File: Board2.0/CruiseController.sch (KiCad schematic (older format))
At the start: 56 parts, among them J1 USB_B_Micro, J2 Conn_02x09_Top_Bottom, U1 ADG884, U3 TLV9064IRTER, U5 MIC5225, U6 MCP2562-E-MF, U7 STM32L433CCUx, Y1 32.768

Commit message: udpate v2 pcb
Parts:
- added R22, R23: 75, Resistor_SMD:R_0603_1608Metric, symbol Device:R_Small
- added U2: CPC1017N, Package_SO:SOP-4_3.8x4.1mm_P2.54mm, symbol Relay_SolidState:CPC1017N
- U1: symbol VeridianDesigns:ADG884 -> CruiseController-rescue:ADG884-VeridianDesigns
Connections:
- net GND: now also J2.11 (Pin_11), U2.2; no longer J2.10 (Pin_10)
- net INTERSW: no longer J2.11 (Pin_11)
- net VIN: no longer J2.1 (Pin_1)
- net HZEN: now reaches U7.16 (PA6)
- net HZEN: now also R22.2
- new net: R23.1, U2.1
- new net: R22.1, R23.2
- new net HZ0: J2.10 (Pin_10), U2.3
- new net HZ1: J2.1 (Pin_1), U2.4
- no-connect marks 21 -> 20
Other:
- note added: "OTHER"
- moved on the sheet: D1, R10, R21, R9, TP1
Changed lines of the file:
@@
 EESchema Schematic File Version 4
 LIBS:CruiseController-cache
-EELAYER 30 0
+EELAYER 29 0
 EELAYER END
 $Descr USLetter 11000 8500
@@
 NoConn ~ 8075 2325
 NoConn ~ 8075 2825
-NoConn ~ 8075 2725
 NoConn ~ 8075 3425
 NoConn ~ 8075 3725
@@
 NoConn ~ 9275 4025
 NoConn ~ 9275 3725
-NoConn ~ 9275 3325
+NoConn ~ 8075 2725
 NoConn ~ 9275 2825
 $Comp
@@
 L Connector:TestPoint TP1
 U 1 1 5DDE6CDB
-P 7150 5475
-F 0 "TP1" H 7208 5593 50  0000 L CNN
-F 1 "TestPoint" H 7208 5502 50  0000 L CNN
-F 2 "TestPoint:TestPoint_THTPad_D1.5mm_Drill0.7mm" H 7350 5475 50  0001 C CNN
-F 3 "~" H 7350 5475 50  0001 C CNN
-	1    7150 5475
+P 9650 4700
+F 0 "TP1" H 9708 4818 50  0000 L CNN
+F 1 "TestPoint" H 9708 4727 50  0000 L CNN
+F 2 "TestPoint:TestPoint_THTPad_D1.5mm_Drill0.7mm" H 9850 4700 50  0001 C CNN
+F 3 "~" H 9850 4700 50  0001 C CNN
+	1    9650 4700
 	1    0    0    -1
 $EndComp
@@
 L power:GND #PWR0105
 U 1 1 5DDE8742
-P 7150 5475
-F 0 "#PWR0105" H 7150 5225 50  0001 C CNN
-F 1 "GND" H 7155 5302 50  0000 C CNN
-F 2 "" H 7150 5475 50  0001 C CNN
-F 3 "" H 7150 5475 50  0001 C CNN
-	1    7150 5475
+P 9650 4700
+F 0 "#PWR0105" H 9650 4450 50  0001 C CNN
+F 1 "GND" H 9655 4527 50  0000 C CNN
+F 2 "" H 9650 4700 50  0001 C CNN
+F 3 "" H 9650 4700 50  0001 C CNN
+	1    9650 4700
 	1    0    0    -1
 $EndComp
@@
 Wire Wire Line
 	1300 1450 1300 1775
-Text GLabel 3350 7425 0    50   Input ~ 0
-VIN
 $Comp
 L power:GND #PWR0106
@@
 Wire Wire Line
 	3850 7025 4525 7025
-$Comp
-L power:GND #PWR0114
-U 1 1 5DF7A588
-P 3850 7425
-F 0 "#PWR0114" H 3850 7175 50  0001 C CNN
-F 1 "GND" H 3855 7252 50  0000 C CNN
-F 2 "" H 3850 7425 50  0001 C CNN
-F 3 "" H 3850 7425 50  0001 C CNN
-	1    3850 7425
-	1    0    0    -1
-$EndComp
 NoConn ~ 8075 3325
 Wire Wire Line
@@
 	1    0    0    -1
 $EndComp
-Text GLabel 3850 7325 2    50   Input ~ 0
-INTERSW
 NoConn ~ 9275 2925
 Text Notes 1725 875  0    157  ~ 31
@@
 MCU
 Wire Notes Line
-	475  6000 10525 6000
-Wire Notes Line
-	10525 6000 10525 5975
+	475  6000 6650 6000
 Wire Notes Line
 	4325 475  4325 6000
@@
 Text Notes 650  6325 0    157  ~ 31
 CONNECTORS
-Wire Notes Line
-	6650 475  6650 6000
 Wire Wire Line
 	5150 4600 5275 4600
@@
 Connection ~ 4425 6400
 $Comp
-L VeridianDesigns:ADG884 U1
+L CruiseController-rescue:ADG884-VeridianDesigns U1
 U 1 1 5DEEE4C5
 P 1950 1675
@@
 $EndComp
 $Comp
-L VeridianDesigns:ADG884 U1
+L CruiseController-rescue:ADG884-VeridianDesigns U1
 U 2 1 5DEEFBA6
 P 2675 3850
@@
 $EndComp
 $Comp
-L VeridianDesigns:ADG884 U1
+L CruiseController-rescue:ADG884-VeridianDesigns U1
 U 3 1 5DEF12DD
 P 2850 4850
@@
 L CruiseController-rescue:155124M173200-VeridianDesigns-CruiseController-rescue D1
 U 1 1 5DF31D3A
-P 8650 5400
-F 0 "D1" H 8650 4973 50  0000 C CNN
-F 1 "155124M173200-VeridianDesigns-CruiseController-rescue" H 8650 5064 50  0000 C CNN
-F 2 "LED_155124M173200" H 8950 5650 50  0001 L BNN
-F 3 "Wurth Electronics" H 8950 5550 50  0001 L BNN
-	1    8650 5400
+P 9225 6175
+F 0 "D1" H 9225 5748 50  0000 C CNN
+F 1 "155124M173200-VeridianDesigns-CruiseController-rescue" H 9225 5839 50  0000 C CNN
+F 2 "LED_155124M173200" H 9525 6425 50  0001 L BNN
+F 3 "Wurth Electronics" H 9525 6325 50  0001 L BNN
+	1    9225 6175
 	-1   0    0    1
 $EndComp
@@
 L Device:R_Small R9
 U 1 1 5DF42CF0
-P 9050 5200
-F 0 "R9" V 8975 5175 50  0000 C CNN
-F 1 "27" V 9050 5200 50  0000 C CNN
-F 2 "Resistor_SMD:R_0603_1608Metric" H 9050 5200 50  0001 C CNN
-F 3 "~" H 9050 5200 50  0001 C CNN
-	1    9050 5200
+P 9625 5975
+F 0 "R9" V 9550 5950 50  0000 C CNN
+F 1 "27" V 9625 5975 50  0000 C CNN
+F 2 "Resistor_SMD:R_0603_1608Metric" H 9625 5975 50  0001 C CNN
+F 3 "~" H 9625 5975 50  0001 C CNN
+	1    9625 5975
 	0    1    1    0
 $EndComp
-Text GLabel 8350 5400 0    50   Input ~ 0
+Text GLabel 8925 6175 0    50   Input ~ 0
 3V3
 $Comp
 L Device:R_Small R10
 U 1 1 5DF44B2A
-P 9050 5400
-F 0 "R10" V 8975 5375 50  0000 C CNN
-F 1 "27" V 9050 5400 50  0000 C CNN
-F 2 "Resistor_SMD:R_0603_1608Metric" H 9050 5400 50  0001 C CNN
-F 3 "~" H 9050 5400 50  0001 C CNN
-	1    9050 5400
+P 9625 6175
+F 0 "R10" V 9550 6150 50  0000 C CNN
+F 1 "27" V 9625 6175 50  0000 C CNN
+F 2 "Resistor_SMD:R_0603_1608Metric" H 9625 6175 50  0001 C CNN
+F 3 "~" H 9625 6175 50  0001 C CNN
+	1    9625 6175
 	0    1    1    0
 $EndComp
@@
 L Device:R_Small R21
 U 1 1 5DF45121
-P 9050 5600
-F 0 "R21" V 8975 5575 50  0000 C CNN
-F 1 "75" V 9050 5600 50  0000 C CNN
-F 2 "Resistor_SMD:R_0603_1608Metric" H 9050 5600 50  0001 C CNN
-F 3 "~" H 9050 5600 50  0001 C CNN
-	1    9050 5600
+P 9625 6375
+F 0 "R21" V 9550 6350 50  0000 C CNN
+F 1 "75" V 9625 6375 50  0000 C CNN
+F 2 "Resistor_SMD:R_0603_1608Metric" H 9625 6375 50  0001 C CNN
+F 3 "~" H 9625 6375 50  0001 C CNN
+	1    9625 6375
 	0    1    1    0
 $EndComp
-Text GLabel 9150 5200 2    50   Input ~ 0
+Text GLabel 9725 5975 2    50   Input ~ 0
 LEDB
-Text GLabel 9150 5400 2    50   Input ~ 0
+Text GLabel 9725 6175 2    50   Input ~ 0
 LEDG
-Text GLabel 9150 5600 2    50   Input ~ 0
+Text GLabel 9725 6375 2    50   Input ~ 0
 LEDR
 Text GLabel 9275 3625 2    50   Input ~ 0
@@
 Text GLabel 8075 4225 0    50   Input ~ 0
 LEDB
+Wire Notes Line
+	10525 5125 6650 5125
+Wire Notes Line
+	6650 475  6650 6775
+Text Notes 6700 5400 0    157  ~ 31
+OTHER
+$Comp
+L Relay_SolidState:CPC1017N U2
+U 1 1 5DFF31F4
+P 7325 6325
+F 0 "U2" H 7325 6650 50  0000 C CNN
+F 1 "CPC1017N" H 7325 6559 50  0000 C CNN
+F 2 "Package_SO:SOP-4_3.8x4.1mm_P2.54mm" H 7125 6125 50  0001 L CIN
+F 3 "http://www.ixysic.com/home/pdfs.nsf/www/CPC1017N.pdf/$file/CPC1017N.pdf" H 7275 6325 50  0001 L CNN
+	1    7325 6325
+	1    0    0    -1
+$EndComp
+$Comp
+L power:GND #PWR02
+U 1 1 5DFF6906
+P 3850 7325
+F 0 "#PWR02" H 3850 7075 50  0001 C CNN
+F 1 "GND" H 3855 7152 50  0000 C CNN
+F 2 "" H 3850 7325 50  0001 C CNN
+F 3 "" H 3850 7325 50  0001 C CNN
+	1    3850 7325
+	0    -1   -1   0
+$EndComp
+Text GLabel 3350 7425 0    50   Input ~ 0
+HZ1
+Text GLabel 3850 7425 2    50   Input ~ 0
+HZ0
+Text GLabel 7625 6425 2    50   Input ~ 0
+HZ0
+Text GLabel 7625 6225 2    50   Input ~ 0
+HZ1
+$Comp
+L power:GND #PWR01
+U 1 1 5DFFB045
+P 7025 6425
+F 0 "#PWR01" H 7025 6175 50  0001 C CNN
+F 1 "GND" H 7030 6252 50  0000 C CNN
+F 2 "" H 7025 6425 50  0001 C CNN
+F 3 "" H 7025 6425 50  0001 C CNN
+	1    7025 6425
+	1    0    0    -1
+$EndComp
+$Comp
+L Device:R_Small R23
+U 1 1 5DFFC7D9
+P 7025 6050
+F 0 "R23" V 6950 6025 50  0000 C CNN
+F 1 "75" V 7025 6050 50  0000 C CNN
+F 2 "Resistor_SMD:R_0603_1608Metric" H 7025 6050 50  0001 C CNN
+F 3 "~" H 7025 6050 50  0001 C CNN
+	1    7025 6050
+	1    0    0    1
+$EndComp
+Wire Wire Line
+	7025 6225 7025 6150
+$Comp
+L Device:R_Small R22
+U 1 1 5E007566
+P 7025 5850
+F 0 "R22" V 6950 5825 50  0000 C CNN
+F 1 "75" V 7025 5850 50  0000 C CNN
+F 2 "Resistor_SMD:R_0603_1608Metric" H 7025 5850 50  0001 C CNN
+F 3 "~" H 7025 5850 50  0001 C CNN
+	1    7025 5850
+	1    0    0    1
+$EndComp
+Text GLabel 7025 5750 1    50   Input ~ 0
+HZEN
+Text GLabel 9275 3325 2    50   Input ~ 0
+HZEN
 $EndSCHEMATC

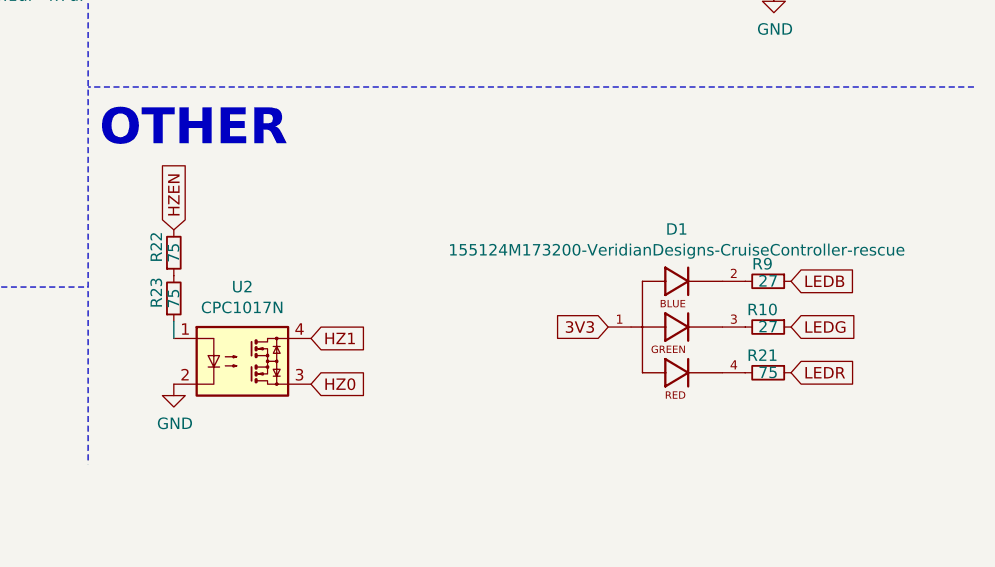
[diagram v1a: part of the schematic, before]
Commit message: pcb v2
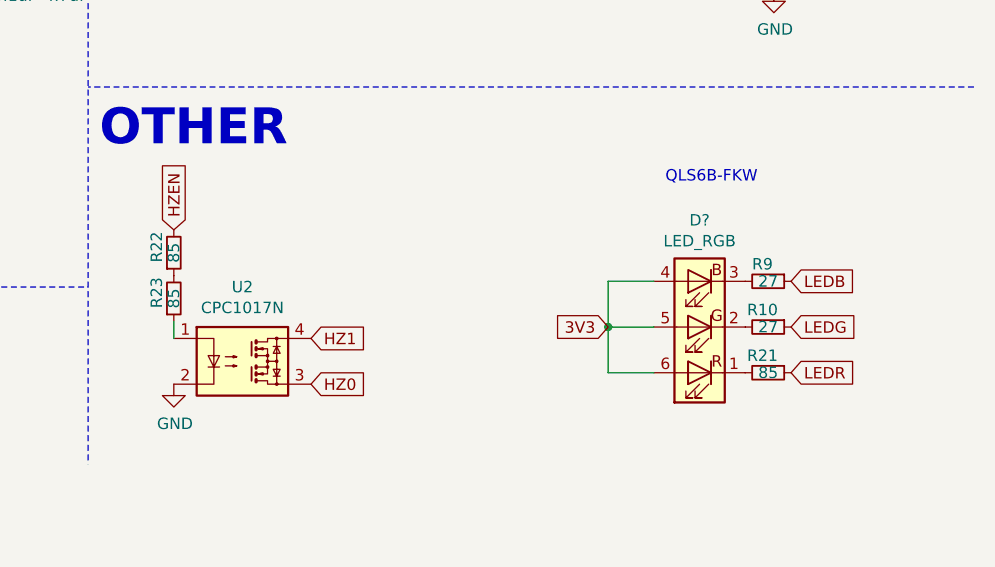
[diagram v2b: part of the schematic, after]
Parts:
- removed D1: 155124M173200-VeridianDesigns-CruiseController-re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, LED_155124M173200, symbol CruiseController-rescue:155124M173200-VeridianDesigns-CruiseController-rescue
- added D?: LED_RGB, symbol Device:LED_RGB
- R21, R22, R23: value 75 -> 85
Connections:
- net 3V3: now also D?.4 (BA), D?.5 (GA), D?.6 (RA)
- net at R9.2: now also D?.3 (BK)
- net at R10.2: now also D?.2 (GK)
- net at R21.2: now also D?.1 (RK)
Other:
- note added: "QLS6B-FKW"
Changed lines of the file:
@@
 	2050 1175 2350 1175
-$Comp
-L CruiseController-rescue:155124M173200-VeridianDesigns-CruiseController-rescue D1
-U 1 1 5DF31D3A
-P 9225 6175
-F 0 "D1" H 9225 5748 50  0000 C CNN
-F 1 "155124M173200-VeridianDesigns-CruiseController-rescue" H 9225 5839 50  0000 C CNN
-F 2 "LED_155124M173200" H 9525 6425 50  0001 L BNN
-F 3 "Wurth Electronics" H 9525 6325 50  0001 L BNN
-	1    9225 6175
-	-1   0    0    1
-$EndComp
 $Comp
 L Device:R_Small R17
@@
 P 9625 6375
 F 0 "R21" V 9550 6350 50  0000 C CNN
-F 1 "75" V 9625 6375 50  0000 C CNN
+F 1 "85" V 9625 6375 50  0000 C CNN
 F 2 "Resistor_SMD:R_0603_1608Metric" H 9625 6375 50  0001 C CNN
 F 3 "~" H 9625 6375 50  0001 C CNN
@@
 P 7025 6050
 F 0 "R23" V 6950 6025 50  0000 C CNN
-F 1 "75" V 7025 6050 50  0000 C CNN
+F 1 "85" V 7025 6050 50  0000 C CNN
 F 2 "Resistor_SMD:R_0603_1608Metric" H 7025 6050 50  0001 C CNN
 F 3 "~" H 7025 6050 50  0001 C CNN
@@
 P 7025 5850
 F 0 "R22" V 6950 5825 50  0000 C CNN
-F 1 "75" V 7025 5850 50  0000 C CNN
+F 1 "85" V 7025 5850 50  0000 C CNN
 F 2 "Resistor_SMD:R_0603_1608Metric" H 7025 5850 50  0001 C CNN
 F 3 "~" H 7025 5850 50  0001 C CNN
@@
 Text GLabel 9275 3325 2    50   Input ~ 0
 HZEN
+$Comp
+L Device:LED_RGB D?
+U 1 1 5DFB533B
+P 9325 6175
+F 0 "D?" H 9325 5708 50  0000 C CNN
+F 1 "LED_RGB" H 9325 5799 50  0000 C CNN
+F 2 "" H 9325 6125 50  0001 C CNN
+F 3 "~" H 9325 6125 50  0001 C CNN
+	1    9325 6175
+	-1   0    0    1
+$EndComp
+Wire Wire Line
+	8925 6175 8925 5975
+Wire Wire Line
+	8925 5975 9125 5975
+Wire Wire Line
+	9125 6175 8925 6175
+Wire Wire Line
+	9125 6375 8925 6375
+Wire Wire Line
+	8925 6375 8925 6175
+Connection ~ 8925 6175
+Text Notes 9175 5550 0    50   ~ 0
+QLS6B-FKW
 $EndSCHEMATC
